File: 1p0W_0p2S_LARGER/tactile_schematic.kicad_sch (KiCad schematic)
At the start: 55 parts, among them IC1 CY8C4145PVI-PS431, J1 Conn_01x03, J2 Conn_01x04, J3 Conn_01x04, J4 Conn_01x03, J5 Conn_ARM_SWD_TagConnect_TC203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

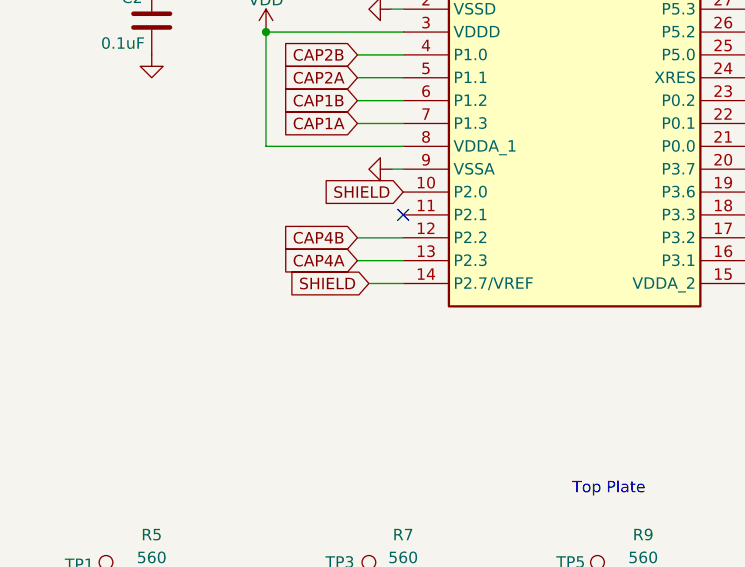
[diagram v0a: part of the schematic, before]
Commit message: more spacing fixes
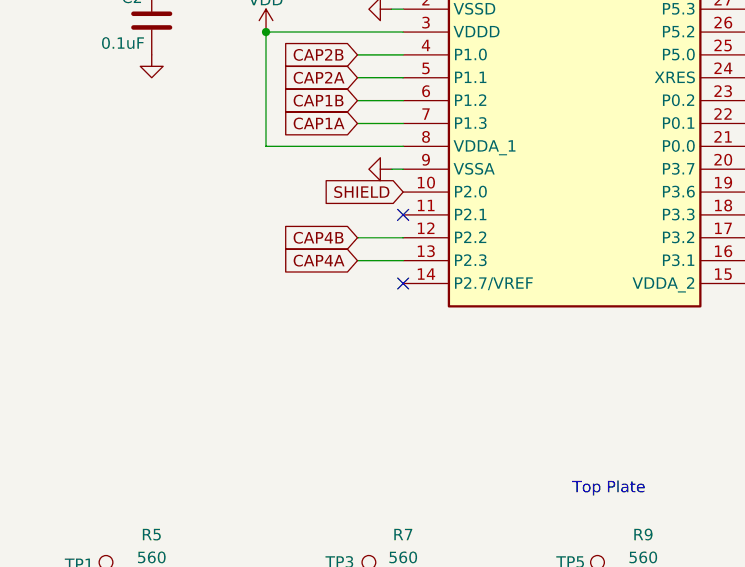
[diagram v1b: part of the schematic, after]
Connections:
- net SHIELD: no longer IC1.14 (P2.7/VREF)
- no-connect marks 10 -> 11
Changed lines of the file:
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@@
+	)
+	(no_connect
+		(at 55.88 62.23)
 	)
 	(no_connect
@@
 	(wire
 		(pts
-			(xy 52.07 62.23) (xy 55.88 62.23)
-		)
-		(stroke
-			(width 0)
-			(type default)
-		)
-	)
-	(wire
-		(pts
 			(xy 93.98 52.07) (xy 97.79 52.07)
 		)
@@
 			(effects
 				(font
-					(size 1.27 1.27)
-				)
-				(justify right)
-				(hide yes)
-			)
-		)
-	)
-	(global_label "SHIELD"
-		(shape input)
-		(at 52.07 62.23 180)
-		(fields_autoplaced yes)
-		(effects
-			(font
-				(size 1.27 1.27)
-			)
-			(justify right)
-		)
-		(property "Intersheetrefs" "${INTERSHEET_REFS}"
-			(at 42.4929 62.23 0)
-			(effects
-				(font
